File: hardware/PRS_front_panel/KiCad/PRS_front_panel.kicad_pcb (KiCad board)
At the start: 2 copper layers, 203 x 51 mm, 0 parts

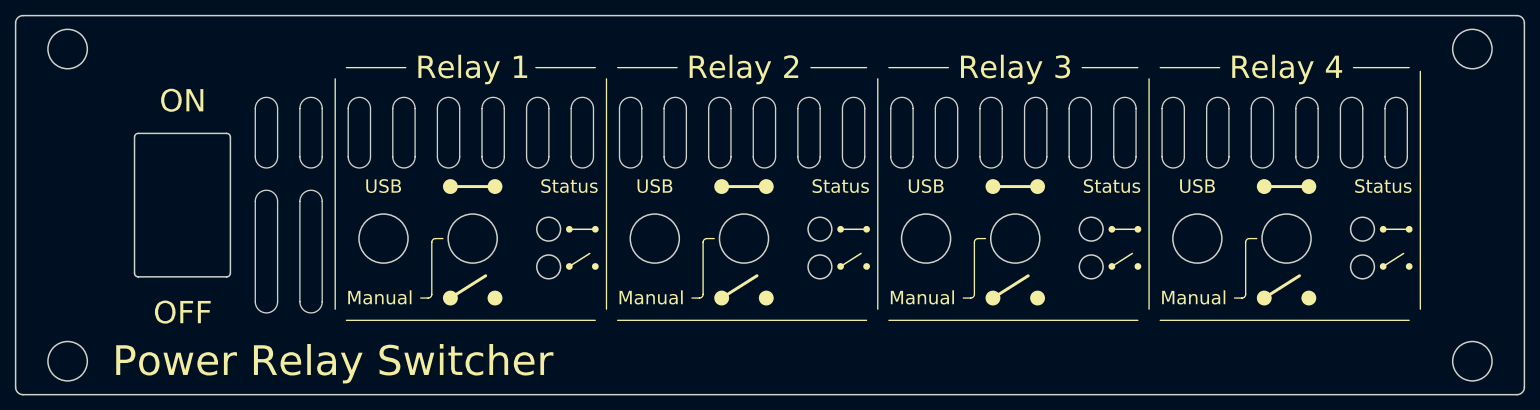
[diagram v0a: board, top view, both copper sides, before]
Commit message: Update PRS_front_panel to KiCad v6
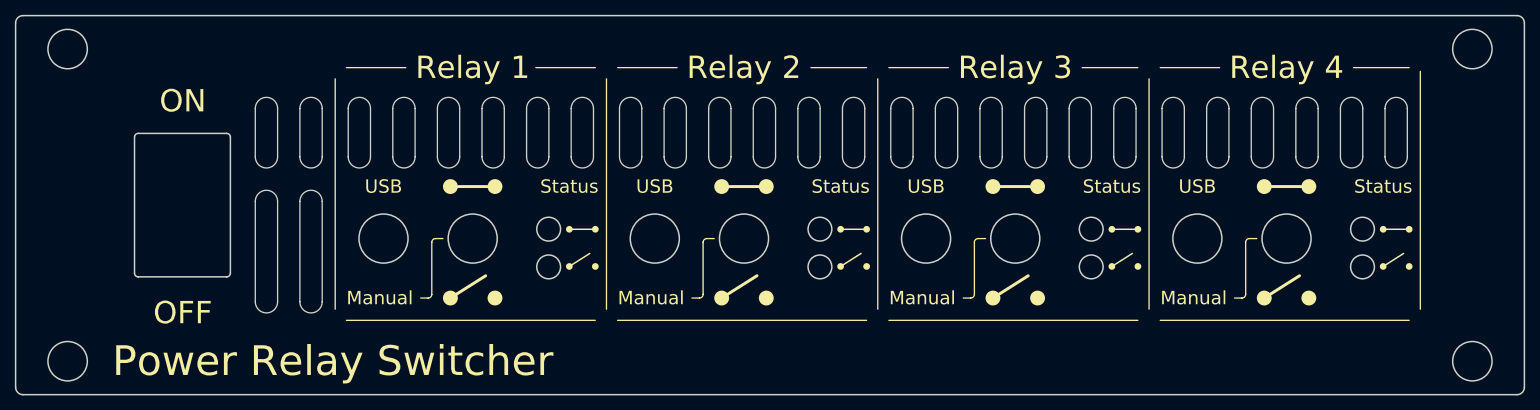
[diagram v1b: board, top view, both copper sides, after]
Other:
- net class Default removed
